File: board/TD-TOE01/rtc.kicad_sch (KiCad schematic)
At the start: 4 parts, among them U9 DS1307, Y2 32.768KHz

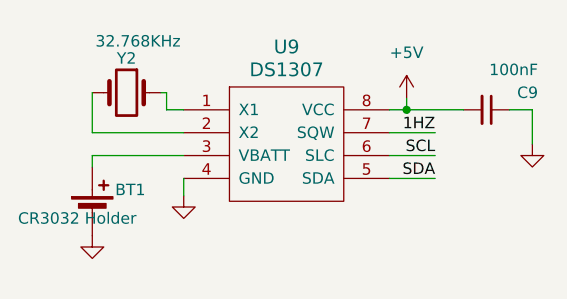
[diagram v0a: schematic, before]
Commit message: OET schematic
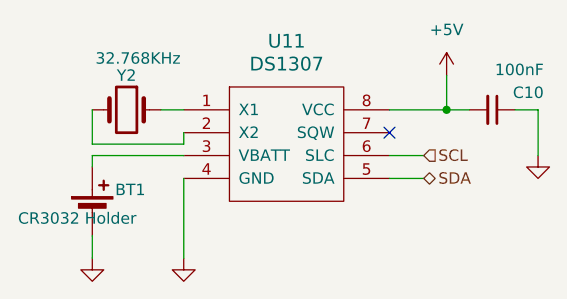
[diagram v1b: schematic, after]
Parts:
- BT1: symbol ClockIt:Battery_Cell -> TokeiDigital:Battery_Cell
- C10: renamed from C9; footprint TokeiDigital:C_0805 -> TokeiDigital:C Rect P5.00; symbol ClockIt:C_Small -> TokeiDigital:C_Small
- U11: renamed from U9; symbol ClockIt:DS1307 -> TokeiDigital:DS1307
- Y2: symbol ClockIt:Crystal -> TokeiDigital:Crystal
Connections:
- net 1HZ: no longer names the net of U11.7 (SQW)
- no-connect marks 0 -> 1
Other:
- moved on the sheet: C10, Y2

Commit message: OET
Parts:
- C10: footprint TokeiDigital:C Rect P5.00 -> TokeiDigital:C_1206
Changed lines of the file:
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@@
 			)
 		)
-		(property "Footprint" "TokeiDigital:C Rect P5.00"
+		(property "Footprint" "TokeiDigital:C_1206"
 			(at 147.32 63.5 0)
 			(effects
